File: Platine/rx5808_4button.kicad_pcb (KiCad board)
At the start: 2 copper layers, 50 parts, among them IC1 ATMEGA328-A, P1 CONN_01X02, P2 CONN_01X05, P4 CONN_01X02, P5 BNC, P6 CONN_01X04, P7 CONN_02X05, U1 TPS62160, U2 RX5808, U3 sn74lvc1g3157, Y1 16 MHz

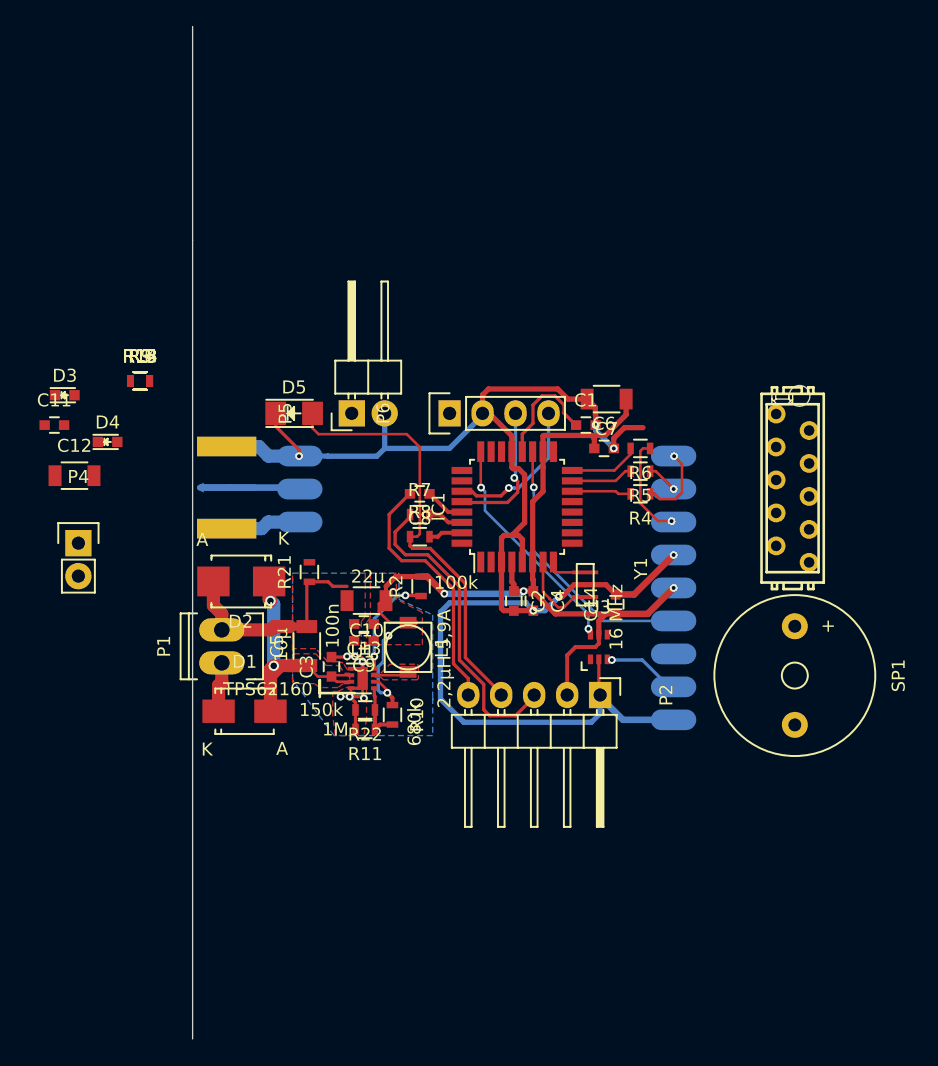
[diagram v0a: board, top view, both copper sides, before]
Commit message: Platine fertig und exportiert.
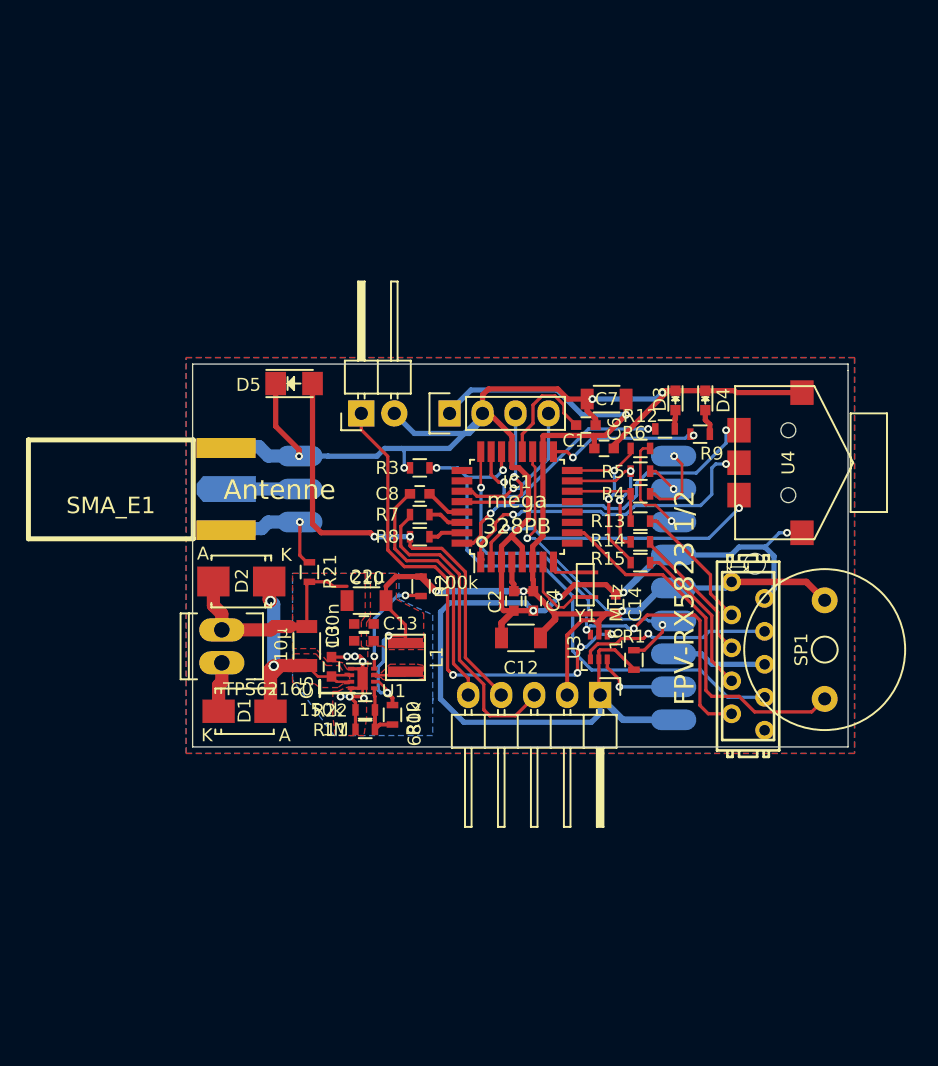
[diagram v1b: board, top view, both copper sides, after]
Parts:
- removed C11: 100n, Capacitors_SMD:C_0603
- removed P4: CONN_01X02, Pin_Headers:Pin_Header_Straight_1x02
- added U4: MCPL3-BC-V, PhilippsFootprints:MCPL3-AC-V, F.Cu at (158.9, 102.6)
- L1: value 2,2µH 5,9A -> 2,2µH 1,5A; footprint TDK_Inductor:VLF4012A -> NR3015:NR3015
- SMA_E1: footprint SMA_EDGE:SMA_EDGE -> PhilippsFootprints:SMA_EDGE_small; moved to F.Cu
- moved D3 47.1 mm to (150.2, 97.8), turned to 270 degrees
- moved D4 46.2 mm to (152.5, 97.8), turned to 270 degrees
- moved R1 43.7 mm to (147.0, 117.8), turned to 270 degrees
- moved R9 43.3 mm to (152.1, 100.4), turned to 180 degrees
- moved R15 41.0 mm to (147.5, 110.3), turned to 180 degrees
- moved R12 40.6 mm to (149.4, 100.0), turned to 180 degrees
- moved R14 40.5 mm to (147.5, 108.7), turned to 180 degrees
- moved R13 40.0 mm to (147.5, 107.1), turned to 180 degrees
- moved C12 36.6 mm to (138.3, 116.1), turned to 180 degrees
- moved R3 22.6 mm to (130.5, 103.0), turned to 180 degrees
- moved P7 13.4 mm to (155.8, 117.5)
- moved SP1 3.05 mm to (161.7, 117.0)
- moved SMA_E1 2.65 mm to (106.7, 105.9)
- moved D5 2.30 mm to (120.8, 96.5)
- moved L1 0.80 mm to (129.4, 117.6)
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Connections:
- SP1 pad 1: /buzzer -> +5V
- SP1 pad 2: GND -> /buzzer
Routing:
- net GND: track 127.1 -> 185.0 mm, vias 6 -> 9
- net /rssi2: track 0.00 -> 43.4 mm, vias 0 -> 2
- net Net-(P5-Pad1): track 0.00 -> 39.3 mm, vias 0 -> 4
- net +5V: track 73.6 -> 106.4 mm, vias 5 -> 6
- net /buzzer: track 0.00 -> 28.9 mm
- net /up: track 0.00 -> 26.8 mm, vias 0 -> 2
- net /mode: track 0.00 -> 25.8 mm, vias 0 -> 2
- net /down: track 0.00 -> 23.4 mm, vias 0 -> 2
- net /led2: track 17.6 -> 39.0 mm, vias 2 -> 3
- net /led1: track 0.00 -> 17.8 mm, vias 0 -> 2
- net /Video2: track 0.00 -> 14.9 mm, vias 0 -> 1
- net /Funk2_clk: track 0.00 -> 12.1 mm
- net /led3: track 0.00 -> 12.0 mm, vias 0 -> 2
- net /Funk2_ss: track 0.00 -> 10.8 mm
- net /Funk2_data: track 0.00 -> 10.1 mm
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- added copper zone on B.Cu, net GND
- added copper zone on F.Cu, net GND
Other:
- board outline added: 50.5 x 29.5 mm
- net class Default: clearance 0.2032 -> 0.2; trace_width 0.3048 -> 0.25
- rule trace_clearance: 0.2032 -> 0.2
- rule trace_min: 0.1524 -> 0.15
- board text added: "328PB"
- board text added: "Antenne"
- board text added: "FPV-RX5823 1/2"
- board text added: "mega"
